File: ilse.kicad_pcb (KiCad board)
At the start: 2 copper layers, 80.9 x 109.5 mm, 87 parts, among them J1 OUT, J2 EURO RACK POWER, J3 CV Inputs, J4 1V/Oct, J5 Gate, J6 Cutoff, J7 Filter In, Q1 BC559, Q2 BC559, Q3 BC559, Q4 BC548, Q5 BC548, Q6 BC548, SW1 LFO to Filter / Freq CV, SW2 Resonance, U1 TL074, U2 TL074

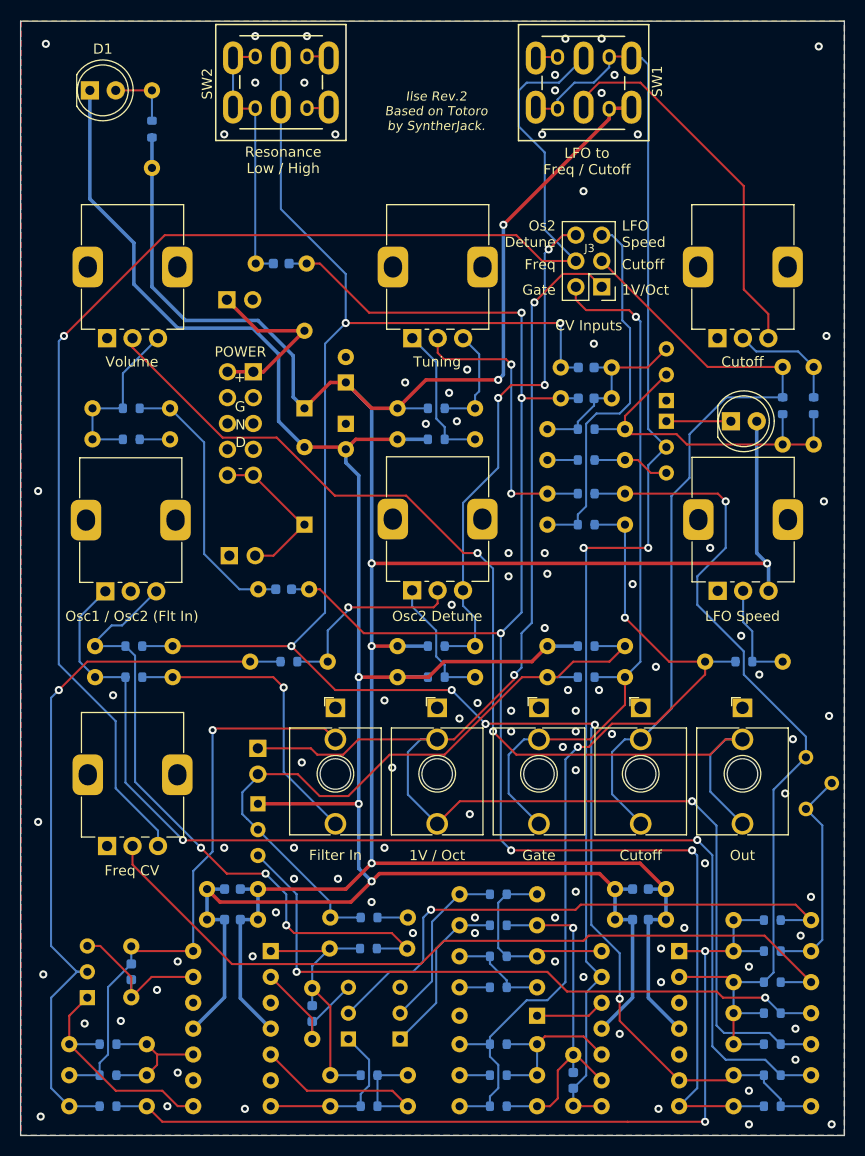
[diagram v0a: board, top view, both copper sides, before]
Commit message: started frontpanel file
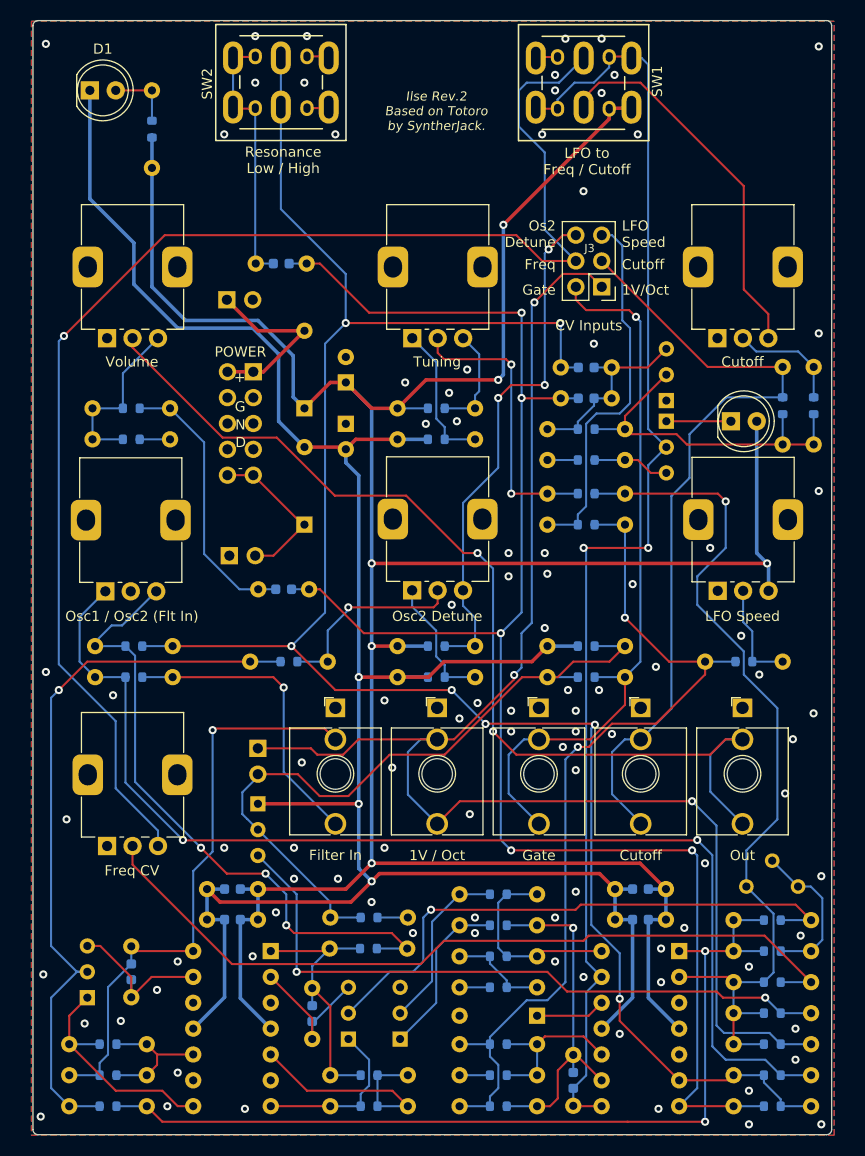
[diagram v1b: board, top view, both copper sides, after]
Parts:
- moved RV3 7.66 mm to (167.7, 121.4), turned to 0 degrees
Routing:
- net Net-(R15-Pad2): track 18.3 -> 11.7 mm
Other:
- board size 80.9 x 109.5 mm -> 78.5 x 109.5 mm
